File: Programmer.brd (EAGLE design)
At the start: 48.3 x 48.3 mm, 32 parts

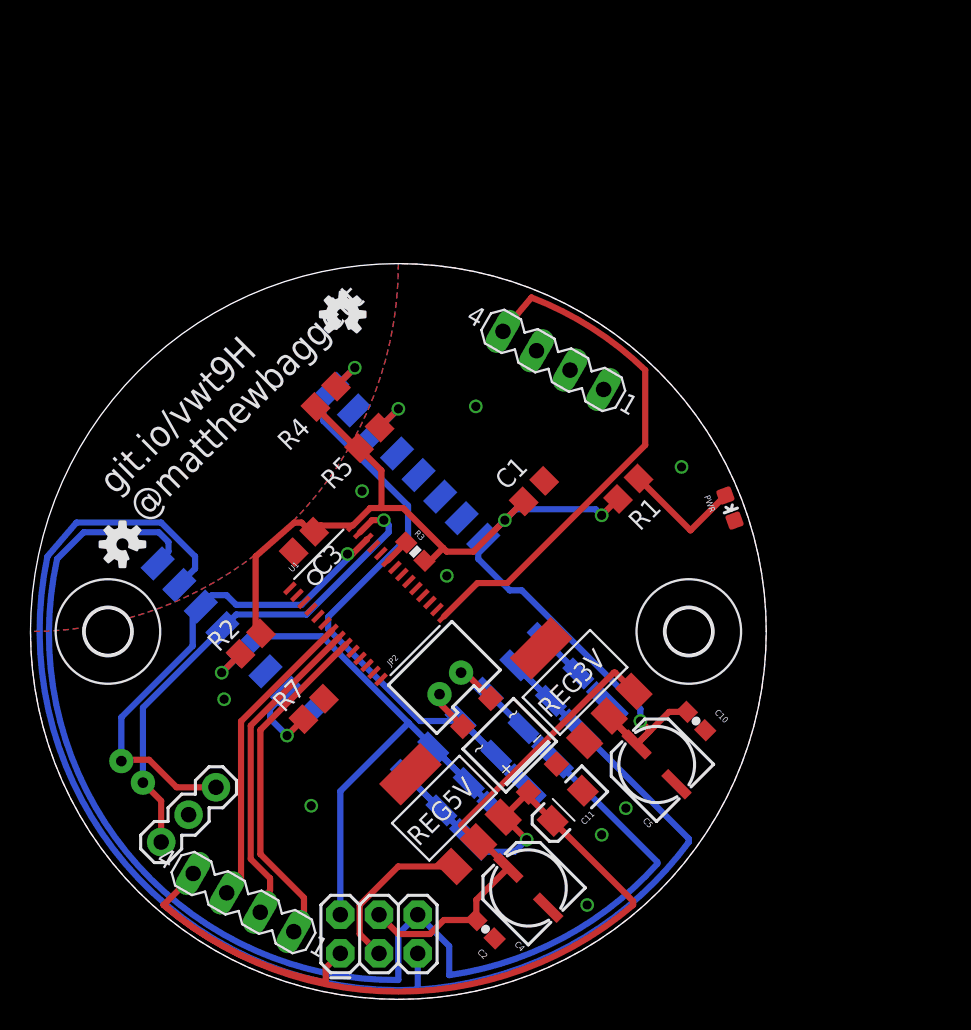
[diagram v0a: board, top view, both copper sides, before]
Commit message: mk9 brah.
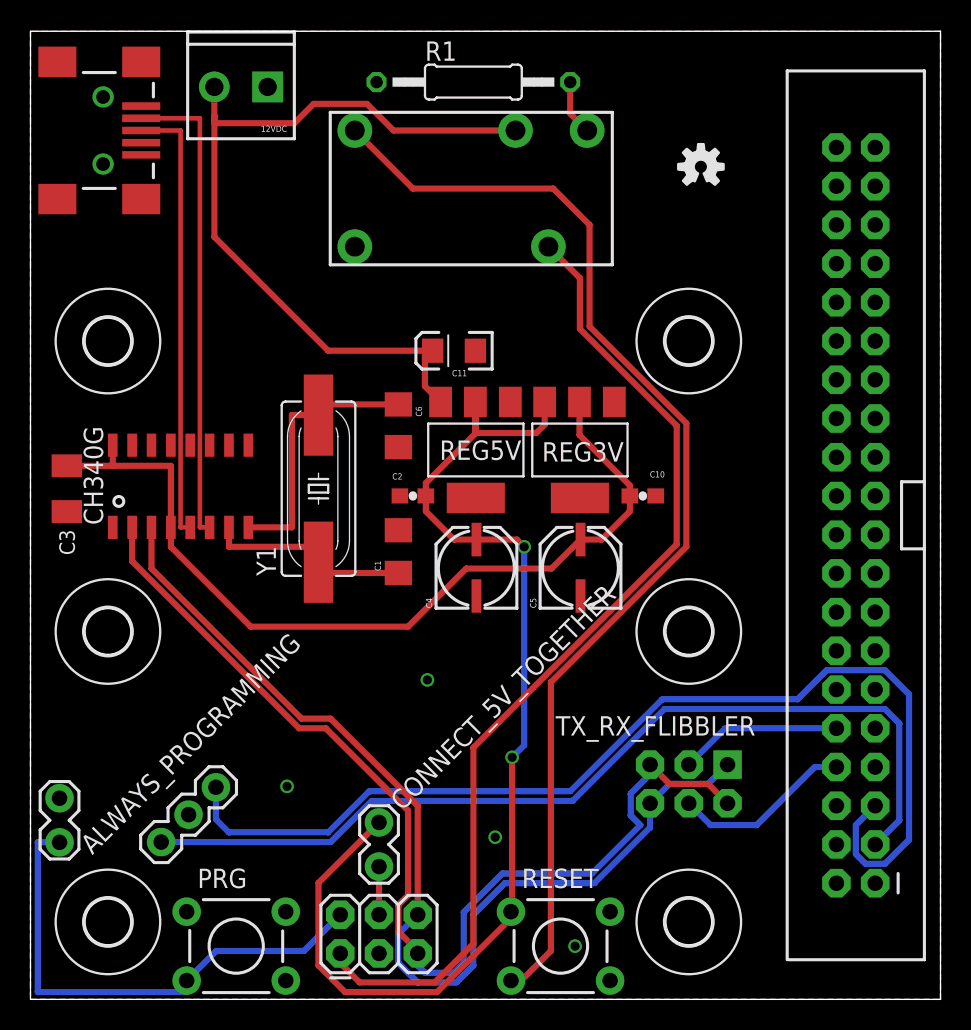
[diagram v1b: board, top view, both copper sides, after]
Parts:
- removed B1: MB1S, rectifier:SOIC-4
- removed I2C1: (no value), SparkFun-Connectors:JST-2-PTH-NS
- removed JP2: (no value), SparkFun-Connectors:JST-2-PTH-VERT
- removed JP3: (no value), SparkFun-Connectors:1X06-SMD_EDGE
- removed LOGO3: OSHW-LOGOS, SparkFun-Aesthetics:OSHW-LOGO-S
- removed PWR: red, SparkFun-LED:LED-0603
- removed R2, R4, R5, R7: 10k, rcl:R0805
- removed R3: (no value), SparkFun-Resistors:0603-RES
- removed SV1, SV2: (no value), con-lstb:MA04-1
- removed U1: (no value), adafruit:TSSOP28
- added 12VDC: (no value), SparkFun-Connectors:SCREWTERMINAL-3.5MM-2
- added ALWAYS_PROGRAMMING, CONNECT_5V_TOGETHER: (no value), SparkFun-Connectors:1X02_LOCK
- added C6: 22pf, SparkFun-Capacitors:1206
- added H3, H4, H5, H6: MOUNT-HOLE3.0, holes:3,0
- added PRG, RESET: SWITCH-MOMENTARY-2PTH, SparkFun-Electromechanical:TACTILE-PTH
- added TX_RX_FLIBBLER: (no value), SparkFun-Connectors:2X3-NS
- added U$2: CH340G, CH340G-USB-SERIAL:SOIC16
- added USB: USB-SMD-NS, SparkFun-Connectors:USB-MINIB-NOSTOP
- added Y1: 12mhz, SparkFun-FreqCtrl:HC49UP
- C1: value 0.1uf -> 22pf; device rcl:C0805 -> SparkFun-Capacitors:1206
- C3: value 0.1uf -> 0.1uF; device rcl:C0805 -> rcl:C1206K
- JP1: value (none) -> RASPBERRYPI-B+-GPIO; device SparkFun-Connectors:1X06_SMD_STRAIGHT_COMBO -> SparkFun-Boards:2X20-SHROUDED
- R1: value 330Ohm -> (none); device rcl:R0805 -> rcl:0207/12
- U$1: value ESP8266_ESP-12 -> RELAYPTH4; device ESP8266-ESP12:ESP8266-ESP12 -> SparkFun-Electromechanical:RELAY-JZC
- moved C11 30.8 mm to (27.8, 42.5), turned to 180 degrees
- moved C2 28.8 mm to (25.1, 33.0), turned to 180 degrees
- moved R1 28.5 mm to (29.1, 60.2), turned to 0 degrees
- moved LOGO2 25.4 mm to (44.0, 54.6)
- moved U$1 24.5 mm to (30.2, 53.2), flipped to the top, turned to 270 degrees
- moved REG5V 23.6 mm to (29.2, 36.0), turned to 180 degrees
- moved JP1 21.4 mm to (54.1, 31.8), flipped to the top, turned to 180 degrees
- moved C4 21.4 mm to (29.1, 28.3), turned to 90 degrees
- moved C3 15.9 mm to (2.38, 33.5), turned to 270 degrees
- moved REG3V 15.2 mm to (36.0, 36.0), turned to 180 degrees
- moved C10 15.2 mm to (40.2, 33.0), turned to 0 degrees
- moved C5 14.0 mm to (35.9, 28.3), turned to 90 degrees
- moved C1 9.74 mm to (24.1, 29.4), turned to 90 degrees
- renumbered JP5 to I2C
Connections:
- removed net #OE: R3.1, U1.23
- removed net ADC: U$1.10
- removed net BLUE: SV1.3, U1.7
- removed net CH_PD: R5.2, U$1.11
- removed net GPIO12: U$1.14
- removed net GPIO13: U$1.15
- removed net GPIO14: U$1.13
- removed net GPIO15: R7.2, U$1.2
- removed net GPIO16: U$1.12
- removed net GPIO2: U$1.3
- removed net GREEN: SV1.1, U1.9
- removed net N$2: PWR.A, R1.1
- removed net N$3: B1.~1, JP2.2
- removed net RED: SV1.2, U1.8
- removed net RESET: JP1.4, JP3.4, R4.2, U$1.9
- removed net WHITE: SV2.4, U1.15
- new net +5V_REMOTE: CONNECT_5V_TOGETHER.2, JP4.4
- new net 12V_REMOTE: JP4.1, U$1.4
- new net NC1: JP1.2
- new net NC2: JP1.4
- new net NC3: JP1.1
- new net NC4: JP1.17
- new net OSCI: C1.1, U$2.7, Y1.1
- new net OSCO: C6.1, U$2.8, Y1.2
- new net RESET_RELAY: RESET.3, U$1.5
- new net RPI_RX: JP1.10, TX_RX_FLIBBLER.3
- new net RPI_TX: JP1.8, TX_RX_FLIBBLER.4
- new net USB_D+: U$2.5, USB.D+
- new net USB_D-: U$2.6, USB.D-
- net +5V: now also CONNECT_5V_TOGETHER.1, RESET.1; no longer JP4.4
- net 12V: now also 12VDC.2, U$1.2; no longer B1.+, JP1.6, JP3.6, JP4.1, SV1.4
- net 3.3V: now also U$2.16, U$2.4; no longer C1.1, R1.2, R2.1, R3.2, R4.1, R5.1, U$1.16, U1.28
- net GND: now also 12VDC.1, ALWAYS_PROGRAMMING.2, C6.2, JP1.14, JP1.20, JP1.25, JP1.30, JP1.34, JP1.39, JP1.6, JP1.9, PRG.1, R1.1, U$2.1, USB.GND; no longer B1.-, JP1.1, JP3.1, PWR.C, R7.1, SV2.1, SV2.2, SV2.3, U1.1, U1.14, U1.2, U1.24, U1.25, U1.3, U1.4, U1.5
- net GPIO0: now also ALWAYS_PROGRAMMING.1, PRG.3; no longer JP1.5, JP3.5, R2.2, U$1.4
- net N$4: now also R1.2, U$1.3; no longer B1.~2, JP2.1
- net RX: now also TX_RX_FLIBBLER.2, TX_RX_FLIBBLER.5, U$2.2; no longer JP1.2, JP3.2, U$1.7
- net SCL: now also JP1.5; no longer I2C1.1, U$1.6, U1.26
- net SDA: now also JP1.3; no longer I2C1.2, U$1.5, U1.27
- net TX: now also TX_RX_FLIBBLER.1, TX_RX_FLIBBLER.6, U$2.3; no longer JP1.3, JP3.3, U$1.8
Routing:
- net RESET_RELAY: track 0.00 -> 75.3 mm
- net 12V_REMOTE: track 0.00 -> 65.7 mm
- net +5V: track 31.8 -> 75.3 mm, vias 0 -> 2
- net RESET: track 41.5 -> 0.00 mm, vias 1 -> 0
- net SCL: track 32.7 -> 70.6 mm, vias 1 -> 0
- net WHITE: track 34.5 -> 0.00 mm
- net USB_D-: track 0.00 -> 31.3 mm
- net USB_D+: track 0.00 -> 29.2 mm
- net SDA: track 33.0 -> 61.0 mm, vias 1 -> 0
- net GREEN: track 22.6 -> 0.00 mm
- net RED: track 21.2 -> 0.00 mm
- net RX: track 90.2 -> 69.7 mm
- net BLUE: track 20.1 -> 0.00 mm
- net 12V: track 72.8 -> 52.8 mm, vias 1 -> 0
- net 3.3V: track 76.0 -> 57.4 mm, vias 3 -> 0
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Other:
- board size 48.3 x 48.3 mm -> 59.7 x 63.5 mm
- board text removed: "@matthewbaggett"
- board text removed: "git.io/vwt9H"
